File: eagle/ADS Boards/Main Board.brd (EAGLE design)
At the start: 61.7 x 61.7 mm, 19 parts, among them J1 62674-121121ALF

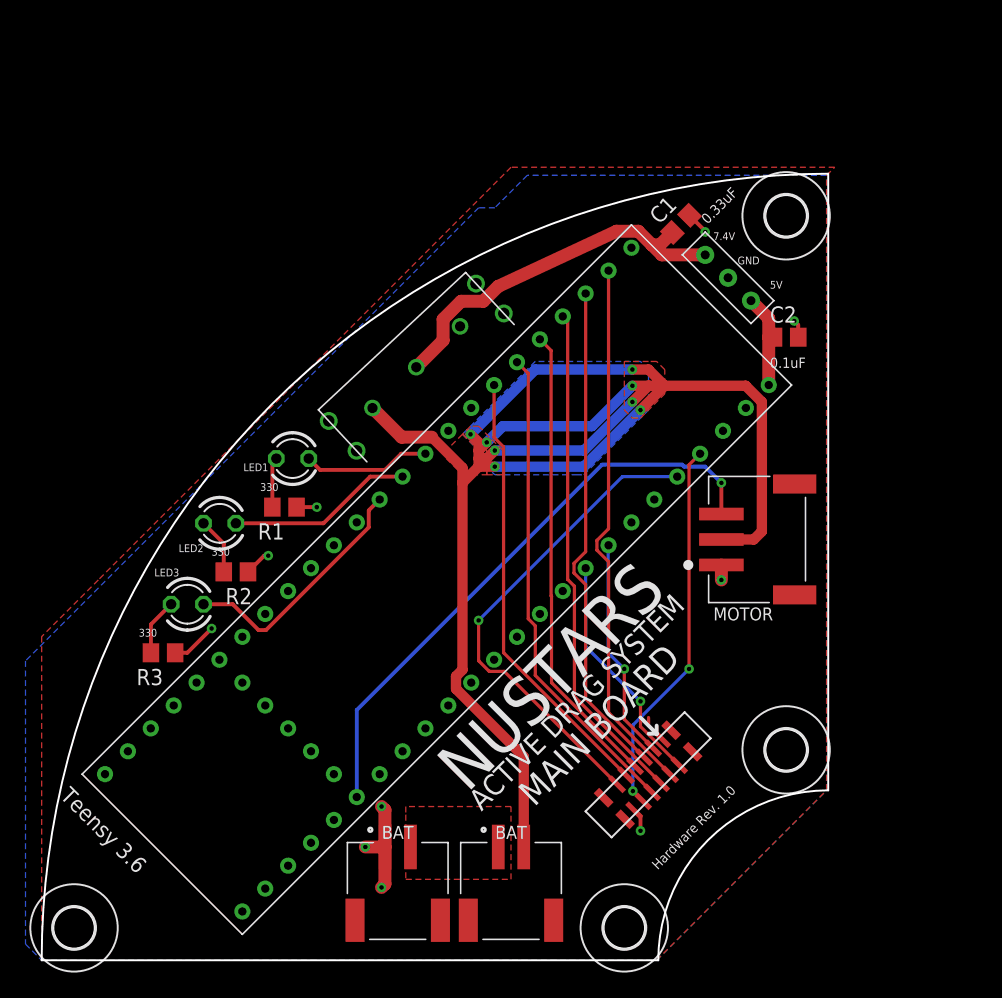
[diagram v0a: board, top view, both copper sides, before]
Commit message: fixed rocket boards
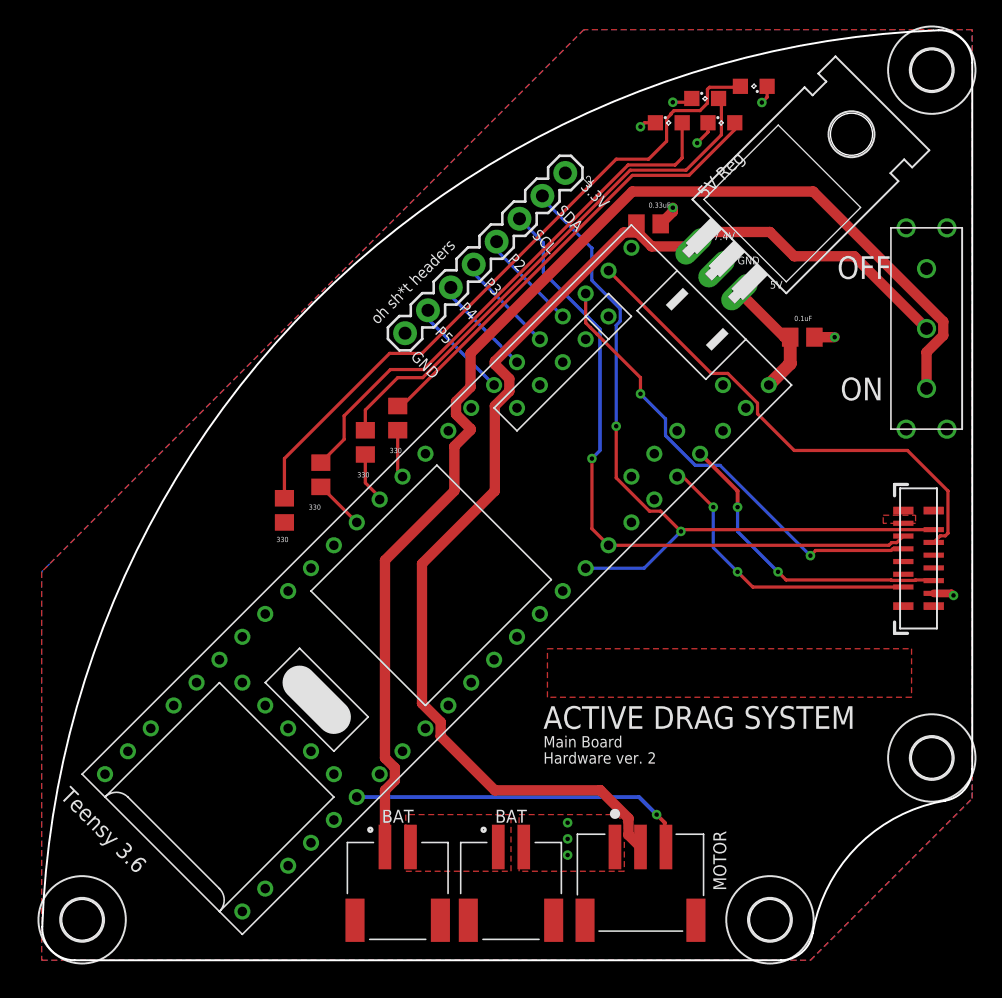
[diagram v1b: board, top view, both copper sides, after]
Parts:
- removed C1: 0.33uF, resistor:C0805
- removed C2: 0.1uF, resistor:C0805
- removed U$2: VREG, NUSTARS ADS Library:VREG
- added C3: 0.33uF, resistor:C0805
- added C4: 0.1uF, resistor:C0805
- added IC1: 7808T, adafruit:TO220H
- added J2: (no value), SparkFun-Connectors:1X08
- added LED4: (no value), led:SML0805
- added R4: 330, resistor:R0805
- LED1, LED2, LED3: device led:LED3MM -> led:SML0805
- moved LED3 56.8 mm to (52.1, 67.6), turned to 0 degrees
- moved LED2 50.4 mm to (53.3, 65.7), turned to 0 degrees
- moved LED1 46.5 mm to (55.9, 68.6)
- moved U$4 40.2 mm to (69.4, 49.6), turned to 270 degrees
- moved J1 28.7 mm to (72.4, 34.3), turned to 90 degrees
- moved MOTOR 25.0 mm to (47.0, 8.89), turned to 180 degrees
- moved R3 22.9 mm to (25.4, 40.6), turned to 270 degrees
- moved R2 17.5 mm to (27.9, 42.5), turned to 270 degrees
- moved H4 16.2 mm to (69.8, 69.8)
- moved H2 11.4 mm to (57.1, 3.17)
- moved H3 11.4 mm to (69.8, 15.9)
- moved H1 0.90 mm to (3.17, 3.17)
- moved R1 0.25 mm to (19.1, 35.3), turned to 270 degrees
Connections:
- removed net N$3: LED2.K, R2.2
- removed net POWER_LED: LED1.A, U$1.P8
- new net MISC_LED: R4.2, U$1.P11
- new net N$5: LED3.A, R3.1
- new net N$6: LED4.A, R4.1
- net 3.3V: now also J2.1, R1.2
- net 5V: now also C4.1, IC1.3; no longer C2.1, U$2.OUTPUT
- net B3: now also J2.4; no longer J1.6
- net B4: now also J2.5; no longer J1.7
- net B5: now also J2.6; no longer J1.8
- net B6: now also J2.7; no longer J1.9
- net ERROR_LED: now also R3.2; no longer LED3.A
- net GND: now also BATTERY1.2, C3.2, C4.2, IC1.2, J2.8, LED1.C, LED2.C, LED3.C, LED4.C; no longer BATTERY2.1, C1.2, C2.2, R1.1, R2.1, R3.1, U$2.GND
- net N$1: now also LED1.A, R1.1; no longer LED1.K, R1.2
- net N$4: now also LED2.A, R2.1; no longer LED3.K, R3.2
- net SCL: now also J2.3
- net SDA: now also J2.2
- net STATUS_LED: now also R2.2; no longer LED2.A
- net V_BATT: now also BATTERY2.1; no longer BATTERY1.2, MOTOR.2
- net V_IN: now also C3.1, IC1.1, MOTOR.2; no longer C1.1, U$2.INPUT
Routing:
- net V_IN: track 30.0 -> 96.2 mm
- net N$1: track 3.94 -> 52.7 mm
- net N$6: track 0.00 -> 42.1 mm
- net SDA: track 18.5 -> 60.2 mm, vias 1 -> 2
- net N$5: track 0.00 -> 41.4 mm
- net V_BATT: track 135.0 -> 95.5 mm, vias 8 -> 0
- net SCL: track 17.4 -> 52.5 mm
- net B3: track 39.8 -> 8.02 mm
- net N$4: track 4.47 -> 36.0 mm
- net B5: track 38.1 -> 8.02 mm
- net B4: track 36.6 -> 8.02 mm
- net B6: track 34.9 -> 8.02 mm
- net MOTOR: track 46.5 -> 26.9 mm
- net ERROR_LED: track 19.7 -> 4.00 mm
- net ADR: track 38.3 -> 23.2 mm, vias 1 -> 2
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- added copper zone on layer 1, net DUMMY
- added copper zone on layer 1, net GND
- removed copper zone on layer 1, net V_BATT
- removed copper zone on layer 16, net V_BATT
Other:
- board size 61.7 x 61.7 mm -> 73 x 73 mm
- board text added: "3.3V"
- board text added: "330"
- board text added: "5V Reg"
- board text added: "C:/Users/ichis/Pictures/NUSTARS Logo PNG.bmp"
- board text added: "Hardware ver. 2"
- board text added: "Main Board"
- board text added: "OFF"
- board text added: "ON"
- board text added: "P2"
- board text added: "P3"
- board text added: "P4"
- board text added: "P5"
- board text added: "R3"
- board text added: "SCL"
- board text added: "SDA"
- board text added: "oh sh*t headers"
- board text removed: "Hardware Rev. 1.0"
- board text removed: "MAIN BOARD"
- board text removed: "NUSTARS"
